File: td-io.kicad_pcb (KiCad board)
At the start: 2 copper layers, 66.5 x 54 mm, 18 parts, among them J1 USB_B, J2 I2C, J3 Dips, J4 Test/Service, J5 Power, J6 Controls, Q1 AO4818B, Q2 AO3400A, U1 ISL3175EIBZ-T, U2 Pico

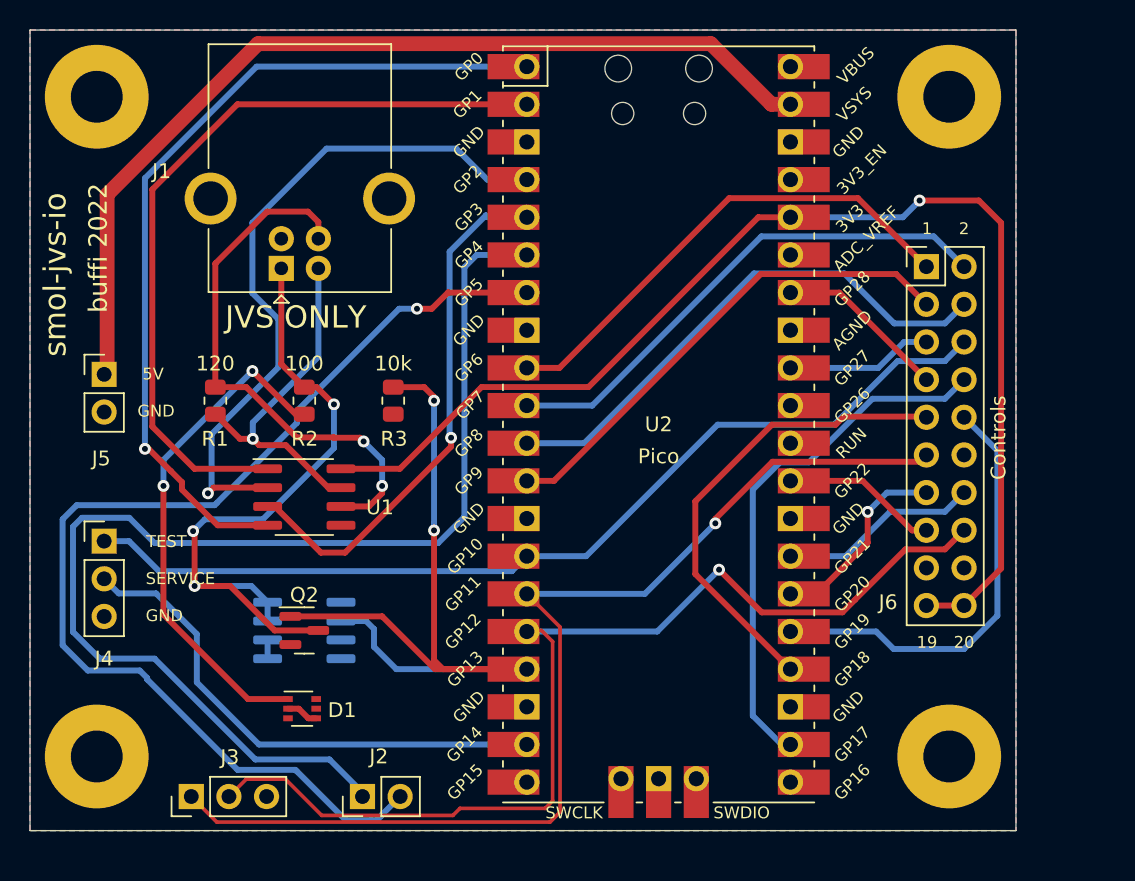
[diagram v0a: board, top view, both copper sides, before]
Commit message: many minor changes
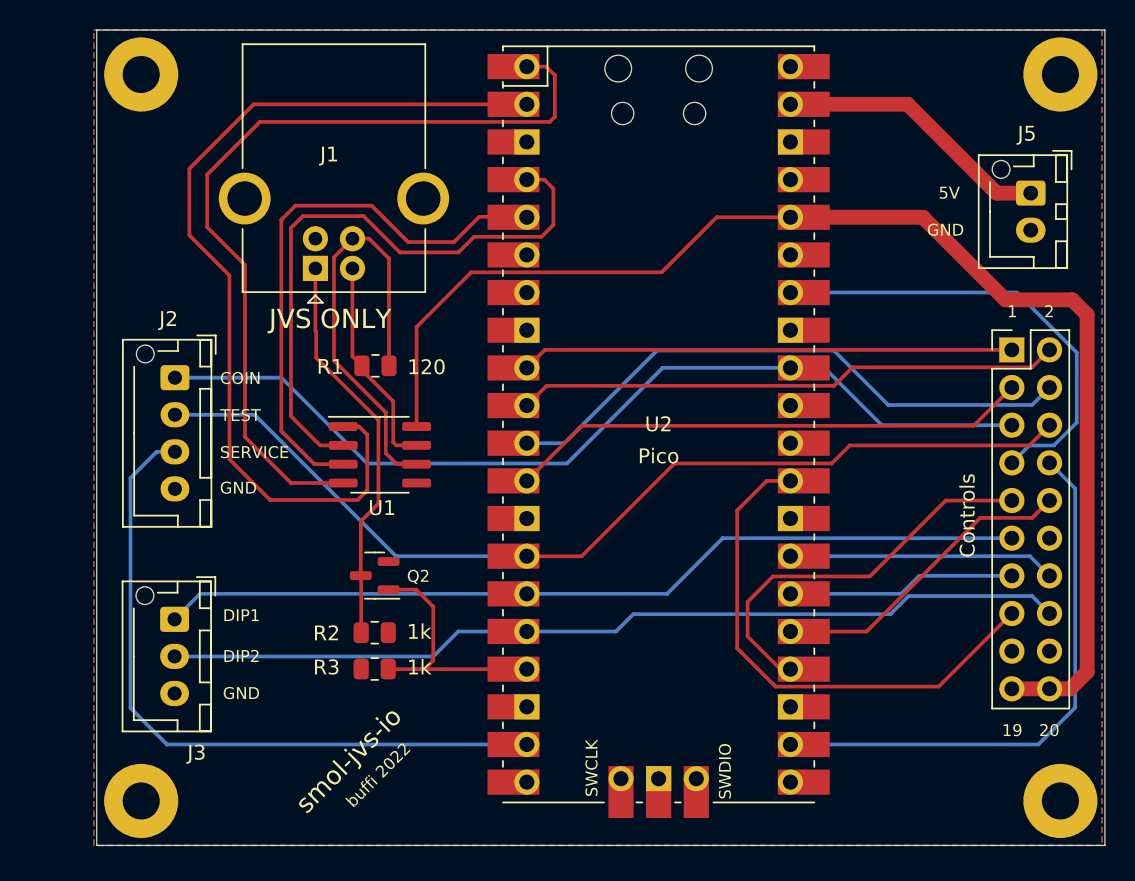
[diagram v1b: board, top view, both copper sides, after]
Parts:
- removed D1: BAV99S, Package_TO_SOT_SMD:SOT-363_SC-70-6
- removed J4: Test/Service, Connector_PinHeader_2.54mm:PinHeader_1x03_P2.54mm_Vertical
- removed Q1: AO4818B, Package_SO:SOIC-8_3.9x4.9mm_P1.27mm
- H1, H2, H3, H4: footprint MountingHole:MountingHole_3.5mm_Pad -> MountingHole:MountingHole_2.5mm_Pad
- J2: value I2C -> Conn_01x04; footprint Connector_PinHeader_2.54mm:PinHeader_1x02_P2.54mm_Vertical -> Connector_JST:JST_XH_B4B-XH-AM_1x04_P2.50mm_Vertical
- J3: footprint Connector_PinHeader_2.54mm:PinHeader_1x03_P2.54mm_Vertical -> Connector_JST:JST_XH_B3B-XH-AM_1x03_P2.50mm_Vertical
- J5: footprint Connector_PinHeader_2.54mm:PinHeader_1x02_P2.54mm_Vertical -> Connector_JST:JST_XH_B2B-XH-AM_1x02_P2.50mm_Vertical
- R2: value 100 -> 1k
- R3: value 10k -> 1k
- moved J5 63.7 mm to (235.0, 55.0), turned to -90 degrees
- moved J2 31.0 mm to (177.3, 67.5), turned to -90 degrees
- moved R3 18.1 mm to (190.8, 87.1), turned to 180 degrees
- moved R2 16.4 mm to (190.8, 84.7), turned to 0 degrees
- moved J3 12.0 mm to (177.2, 83.8), turned to -90 degrees
- moved R1 11.1 mm to (190.8, 66.7), turned to 180 degrees
- moved H4 8.08 mm to (237.0, 96.0)
- moved J6 8.05 mm to (233.7, 65.6)
- moved H2 7.65 mm to (237.0, 47.0)
- moved Q2 6.02 mm to (190.8, 80.8), turned to 180 degrees
- moved U1 5.84 mm to (191.1, 72.7)
- moved H3 4.24 mm to (175.0, 96.0)
- moved H1 3.35 mm to (175.0, 47.0)
- moved J1 2.30 mm to (186.8, 60.1)
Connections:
- H1 pad 1: GND -> unconnected-(H1-Pad1)
- H2 pad 1: GND -> unconnected-(H2-Pad1)
- H3 pad 1: GND -> unconnected-(H3-Pad1)
- H4 pad 1: GND -> unconnected-(H4-Pad1)
- J2 pad 1: Net-(J2-Pad1) -> /b_coin
- J2 pad 2: Net-(J2-Pad2) -> /b_test
- R2 pad 2: Net-(D1-Pad1) -> GND
- U2 pad 6: Net-(J2-Pad1) -> unconnected-(U2-Pad6)
- U2 pad 7: Net-(J2-Pad2) -> unconnected-(U2-Pad7)
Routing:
- net Net-(J2-Pad1): track 80.9 -> 0.00 mm
- net Net-(J2-Pad2): track 75.0 -> 0.00 mm, vias 1 -> 0
- net /b_coin: track 9.89 -> 63.1 mm
- net +5V: track 64.2 -> 18.7 mm
- net /sense_0v: track 59.3 -> 17.3 mm, vias 2 -> 0
- net Net-(D1-Pad1): track 34.4 -> 0.00 mm, vias 2 -> 0
- net /b_6: track 10.6 -> 35.4 mm
- net /b_start: track 11.6 -> 31.2 mm
- net /jvs_sense: track 45.9 -> 26.8 mm, vias 3 -> 0
- net /dip1: track 72.5 -> 58.7 mm, vias 1 -> 0
- net /b_service: track 35.0 -> 47.0 mm
- net /dip2: track 71.3 -> 61.2 mm, vias 1 -> 0
- net Net-(J1-Pad2): track 23.9 -> 14.5 mm, vias 1 -> 0
- net /jvs_rx: track 52.6 -> 61.6 mm
- net /b_3: track 29.7 -> 21.1 mm
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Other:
- board size 66.5 x 54 mm -> 68 x 55 mm
- board text added: "COIN"
- board text added: "DIP1"
- board text added: "DIP2"
- board text removed: "Alternative footprint"
